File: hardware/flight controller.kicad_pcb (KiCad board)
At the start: 4 copper layers, 50.2 x 98.1 mm, 98 parts, among them J1 Input Power, J10 M8, J11 M9, J12 M10, J13 M11, J14 M12, J15 I2C4, J16 Video In, J17 Video Out, J18 LED Strip, J19 USB_C_Receptacle_USB2.0_16P, J2 M1, J20 UART2, J21 UART7, J22 UART5, J23 UART8, J24 GPIO, J25 SWD, J26 UART3, J27 UART4, J3 M2, J4 M3, J5 M4, J6 M5, J7 M6, J8 Micro_SD_Card, J9 M7, U1 TPS54302, U2 BMP388, U3 QMC5883P, U4 STM32H743VITx, U5 AT7456E, U6 ICM-42688-P, Y1 Crystal_GND24, Y3 32.768kHz, Y4 16MHz

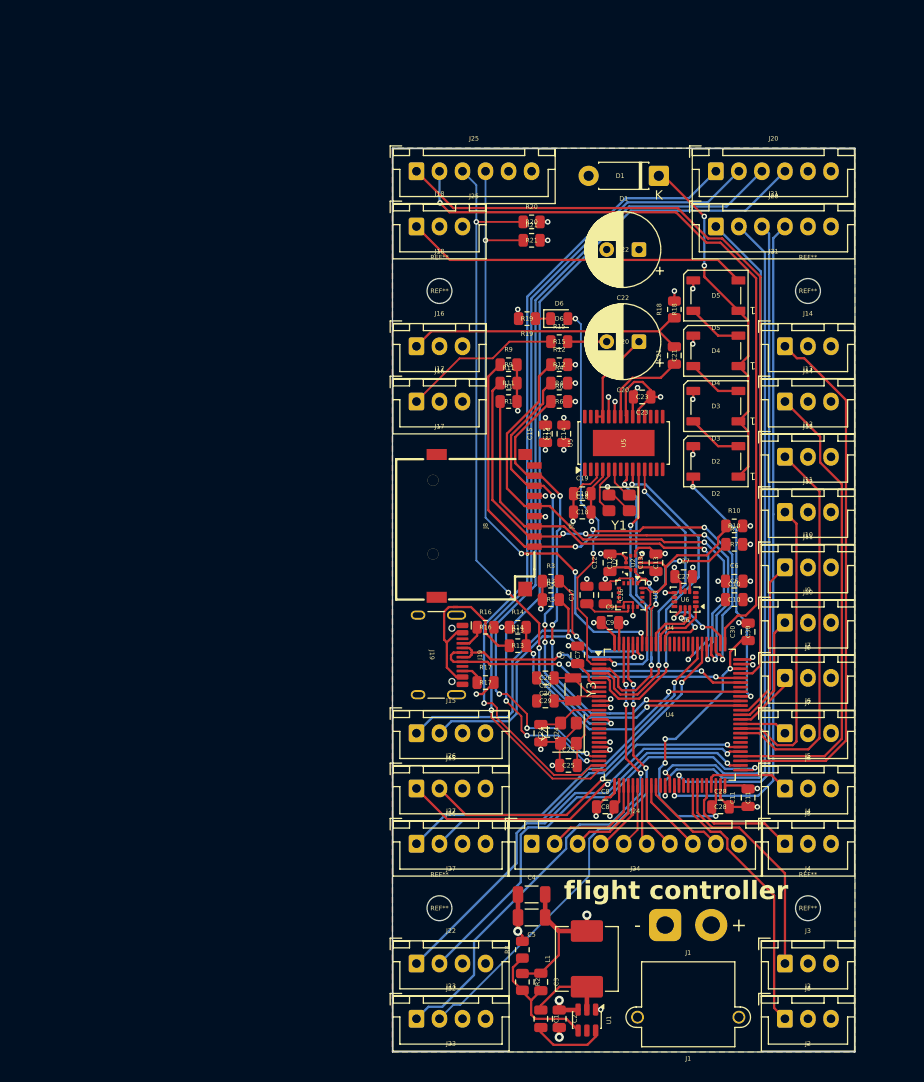
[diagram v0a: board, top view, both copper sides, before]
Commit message: smol
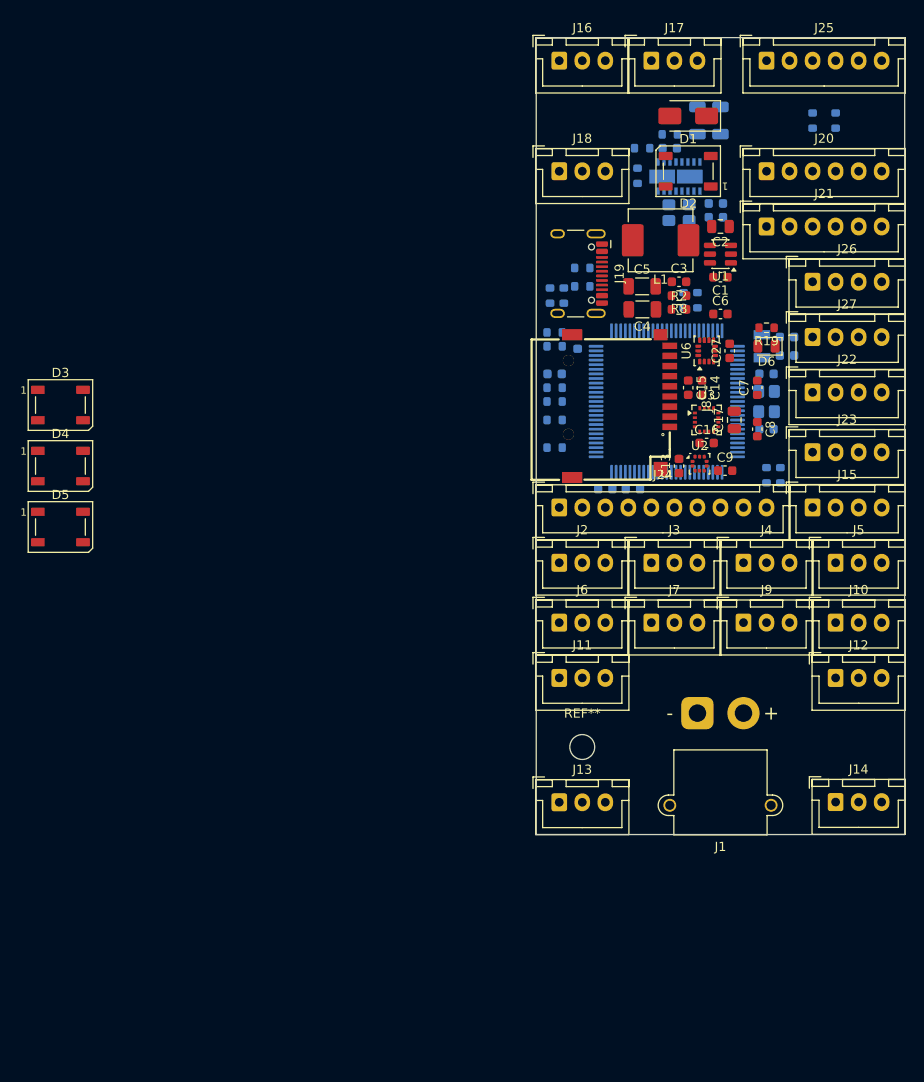
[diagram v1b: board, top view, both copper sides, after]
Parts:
- removed C12, C19, C21, C23: 100nF, Capacitor_SMD:C_0805_2012Metric
- removed C18: 1uF, Capacitor_SMD:C_0805_2012Metric
- removed C20: 470uF, Capacitor_THT:CP_Radial_D8.0mm_P3.50mm
- removed C22: 1000uF, Capacitor_THT:CP_Radial_D8.0mm_P3.50mm
- removed R15, R18: 75, Resistor_SMD:R_0805_2012Metric
- removed the REF** at (167.0, 78.5)
- removed the REF** at (167.0, 145.5)
- removed the REF** at (127.0, 145.5)
- removed the REF** at (127.0, 78.5)
- removed U5: AT7456E, Package_SO:TSSOP-28-1EP_4.4x9.7mm_P0.65mm_EP2.85x6.7mm
- removed Y1: Crystal_GND24, Crystal:Crystal_SMD_3225-4Pin_3.2x2.5mm
- added C31: 22uF, Capacitor_SMD:C_1206_3216Metric, B.Cu at (157.5, 60.0)
- added C32: 22uF, Capacitor_SMD:C_1206_3216Metric, B.Cu at (155.0, 60.0)
- added C33: 100nF, Capacitor_SMD:C_0603_1608Metric, B.Cu at (152.0, 63.0)
- added C34: 100nF, Capacitor_SMD:C_0603_1608Metric, B.Cu at (157.0, 69.0)
- added C35: 1uF, Capacitor_SMD:C_0603_1608Metric, B.Cu at (157.0, 70.5)
- added R22: 1K, Resistor_SMD:R_0603_1608Metric, B.Cu at (148.5, 66.0)
- added R23: 75, Resistor_SMD:R_0603_1608Metric, B.Cu at (152.0, 61.5)
- added R24: 75, Resistor_SMD:R_0603_1608Metric, B.Cu at (149.0, 63.0)
- added REF**: MountingHole_2.7mm_M2.5, MountingHole:MountingHole_2.7mm_M2.5, F.Cu at (142.5, 128.0)
- added U7: AT7456ELAH_C42388749, lcsc:LGA-16_L6.8-W4.0-P0.65-TL-2EP, B.Cu at (153.0, 66.1)
- added Y2: Crystal_GND24, Crystal:Crystal_SMD_3225-4Pin_3.2x2.5mm, B.Cu at (153.0, 70.0)
- C1, C13, C14, C15, C16, C27, C3, C6, C7, C8, C9: footprint Capacitor_SMD:C_0805_2012Metric -> Capacitor_SMD:C_0603_1608Metric
- C10, C11, C24, C25, C26, C28, C29, C30: footprint Capacitor_SMD:C_0805_2012Metric -> Capacitor_SMD:C_0603_1608Metric; moved to B.Cu
- D1: value 1N4001 -> SS54; footprint Diode_THT:D_DO-41_SOD81_P7.62mm_Horizontal -> Diode_SMD:D_SMA
- R1, R10, R11, R12, R13, R14, R16, R17, R20, R21, R3, R4, R5, R6, R7, R9: footprint Resistor_SMD:R_0805_2012Metric -> Resistor_SMD:R_0603_1608Metric; moved to B.Cu
- R19, R2, R8: footprint Resistor_SMD:R_0805_2012Metric -> Resistor_SMD:R_0603_1608Metric
- U4, Y3, Y4: moved to B.Cu
- moved C2 87.8 mm to (157.5, 71.5), turned to 180 degrees
- moved U1 84.4 mm to (157.5, 74.5), turned to 180 degrees
- moved C1 82.8 mm to (157.5, 77.0), turned to 180 degrees
- moved L1 78.4 mm to (151.0, 73.0), turned to 180 degrees
- moved C3 77.5 mm to (153.0, 77.5), turned to 0 degrees
- moved J22 75.5 mm to (167.5, 89.5)
- moved D5 75.4 mm to (85.9, 104.1), turned to 0 degrees
- moved J23 75.0 mm to (167.5, 96.0)
- moved R2 75.0 mm to (153.0, 80.5), turned to 0 degrees
- moved R8 73.0 mm to (153.0, 79.0), turned to 180 degrees
- moved D4 72.2 mm to (85.9, 97.5), turned to 0 degrees
- moved D3 71.1 mm to (85.9, 90.9), turned to 0 degrees
- moved J26 69.8 mm to (167.5, 77.5)
- moved J27 69.8 mm to (167.5, 83.5)
- moved C5 69.5 mm to (149.0, 78.0), turned to 0 degrees
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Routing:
- net +3.3V: track 91.6 -> 0.00 mm, vias 28 -> 0
- net /UART2_RTS: track 91.0 -> 0.00 mm, vias 3 -> 0
- net /UART2_RX: track 90.3 -> 0.00 mm, vias 1 -> 0
- net /UART2_CTS: track 89.6 -> 0.00 mm, vias 3 -> 0
- net /UART2_TX: track 89.0 -> 0.00 mm, vias 1 -> 0
- net /SWDIO: track 86.8 -> 0.00 mm
- net /SWCLK: track 82.8 -> 0.00 mm, vias 1 -> 0
- net GND: track 81.8 -> 0.00 mm, vias 37 -> 0
- net /UART7_RX: track 75.1 -> 0.00 mm, vias 1 -> 0
- net /NRST: track 74.6 -> 0.00 mm, vias 4 -> 0
- net /UART7_TX: track 73.8 -> 0.00 mm, vias 1 -> 0
- net /UART7_RTS: track 73.4 -> 0.00 mm, vias 1 -> 0
- net /UART7_CTS: track 71.8 -> 0.00 mm, vias 1 -> 0
- net /BOOT0: track 67.7 -> 0.00 mm, vias 4 -> 0
- net /SD_D2: track 60.9 -> 0.00 mm, vias 4 -> 0
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- removed copper zone on In2.Cu, net +3.3V
- removed copper zone on In2.Cu, net +5V
- removed copper zone on B.Cu, net GND
- removed copper zone on F.Cu, net GND
- removed copper zone on In1.Cu, net GND
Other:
- board size 50.2 x 98.1 mm -> 40 x 86.5 mm
- board text removed: "flight controller"
